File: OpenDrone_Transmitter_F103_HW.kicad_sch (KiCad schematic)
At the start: 75 parts, among them J1 Conn_01x03, J10 Conn_01x04, J11 Conn_01x03, J12 Conn_01x04, J13 Conn_01x02, J14 Conn_01x05, J15 Conn_01x02, J16 Conn_02x04_Odd_Even, J17 Conn_01x02, J18 Conn_01x02, J19 Conn_01x03, J2 Conn_01x05, J20 Conn_01x02, J21 Conn_01x02, J22 Conn_01x02, J3 Conn_01x03, J4 Conn_01x03, J5 Conn_01x03, J6 Conn_01x02, J7 Conn_01x02, J8 Conn_01x03, J9 Conn_01x03, SW1 RESET, U1 STM32F103C8Tx, U2 AMS1117-3.3, U3 TPS54331, Y2 Crystal_GND24

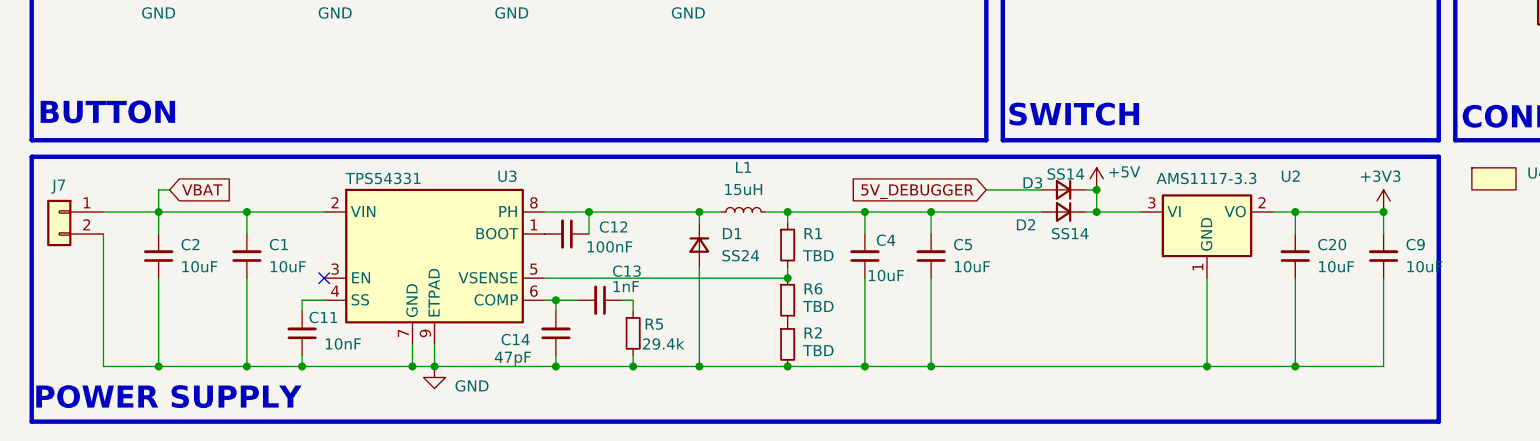
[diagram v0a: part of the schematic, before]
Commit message: update project
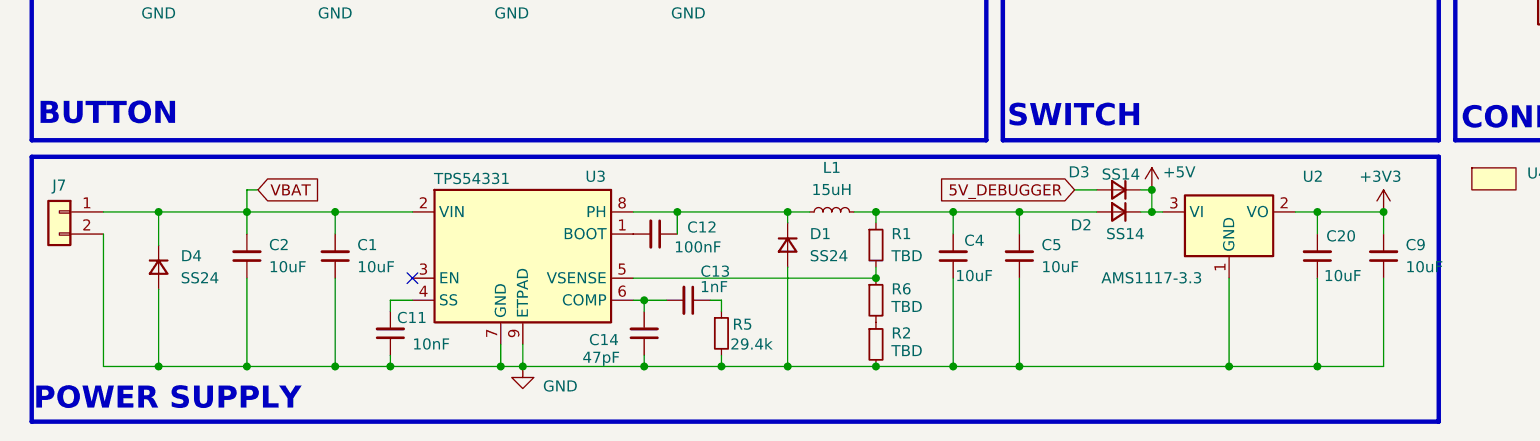
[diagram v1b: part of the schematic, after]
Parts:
- added D4: SS24, Diode_SMD:D_SMA, symbol Device:D_Small
- J10, J12: footprint Footprint:Connector_XH_1x04_P1.25mm_Horizontal -> Footprint:Connector_XH_1x04_P1.25mm_Vertical
- J14, J2: footprint Footprint:Connector_XH_1x05_P1.25mm_Horizontal -> Footprint:Connector_XH_1x05_P1.25mm_Vertical
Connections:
- net GND: now also D4.2 (A)
- net VBAT: now also D4.1 (K)
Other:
- moved on the sheet: C1, C11, C12, C13, C14, C2, C20, C4, C5, D1, D2, D3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
